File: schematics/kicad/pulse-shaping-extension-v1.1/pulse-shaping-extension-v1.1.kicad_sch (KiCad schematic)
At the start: 86 parts, among them J1 Conn_02x10_Odd_Even, J2 Conn_Coaxial, J3 Conn_Coaxial, J4 Conn_01x02_Pin, J5 Conn_01x02_Pin, J6 Conn_01x03_Pin, J7 Conn_Coaxial, U1 AD9102BCPZRL7, U2 ADM8829ARTZ-REEL7, U3 ADA4817-1ACP, U4 THS3091DDAR, X1 OB3225125MLDB6SI-00

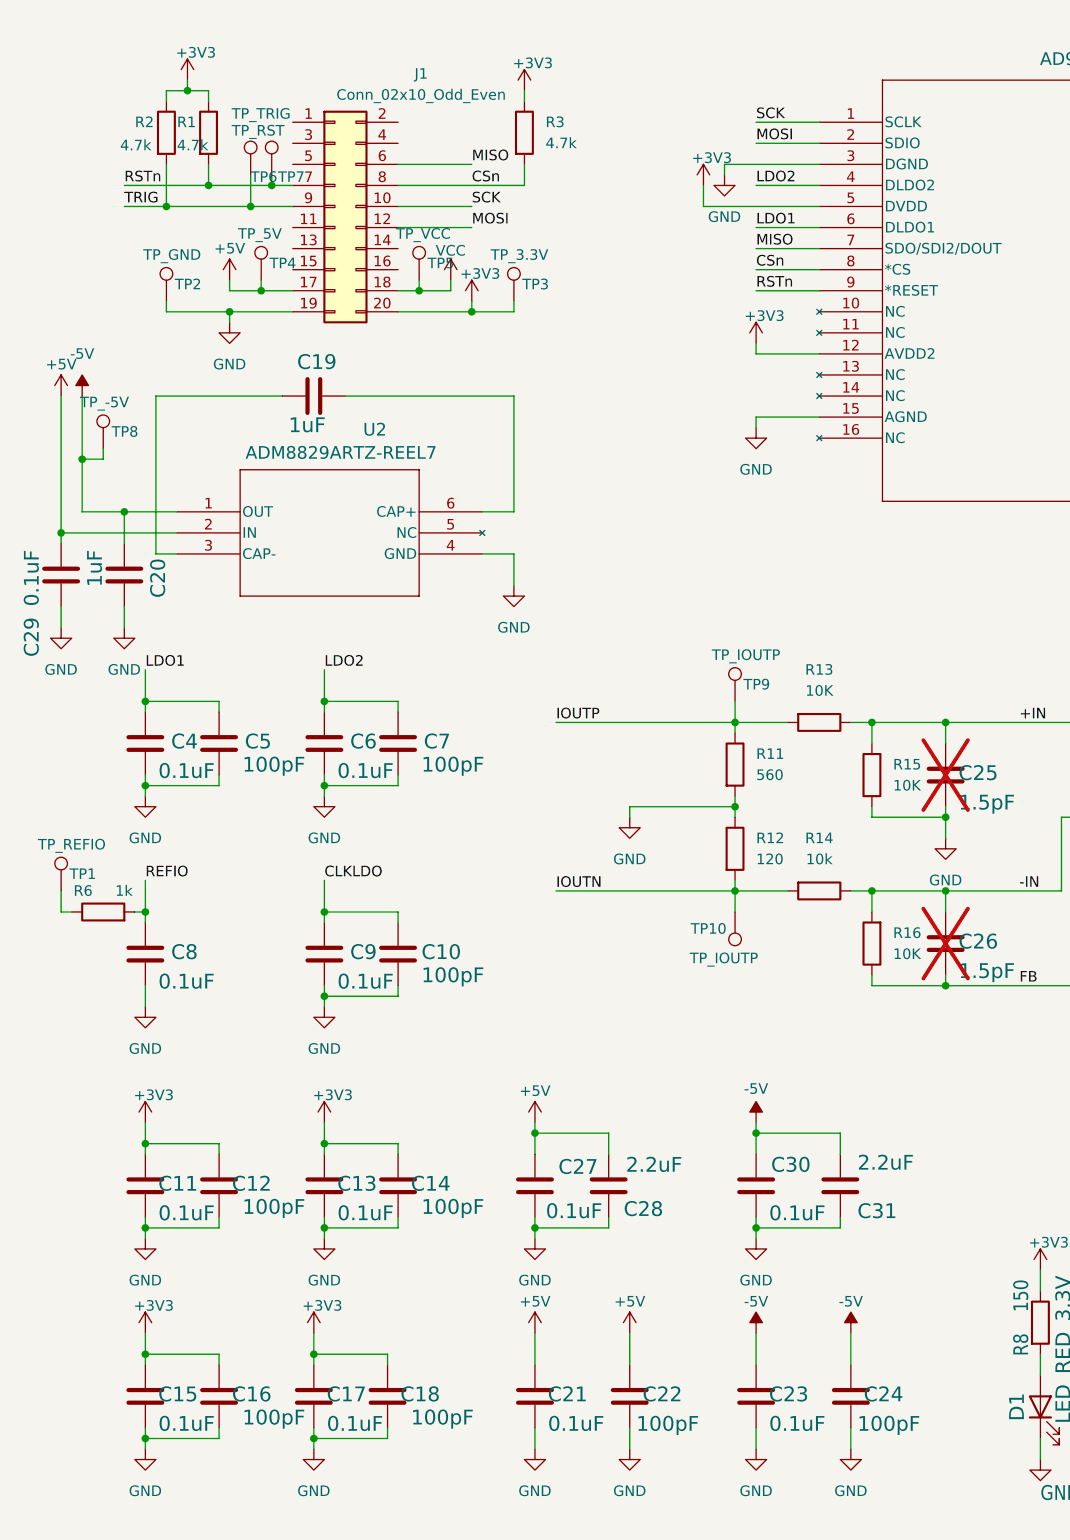
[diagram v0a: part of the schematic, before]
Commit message: Replaced dc-dc converter in pulse shaping expansion board.
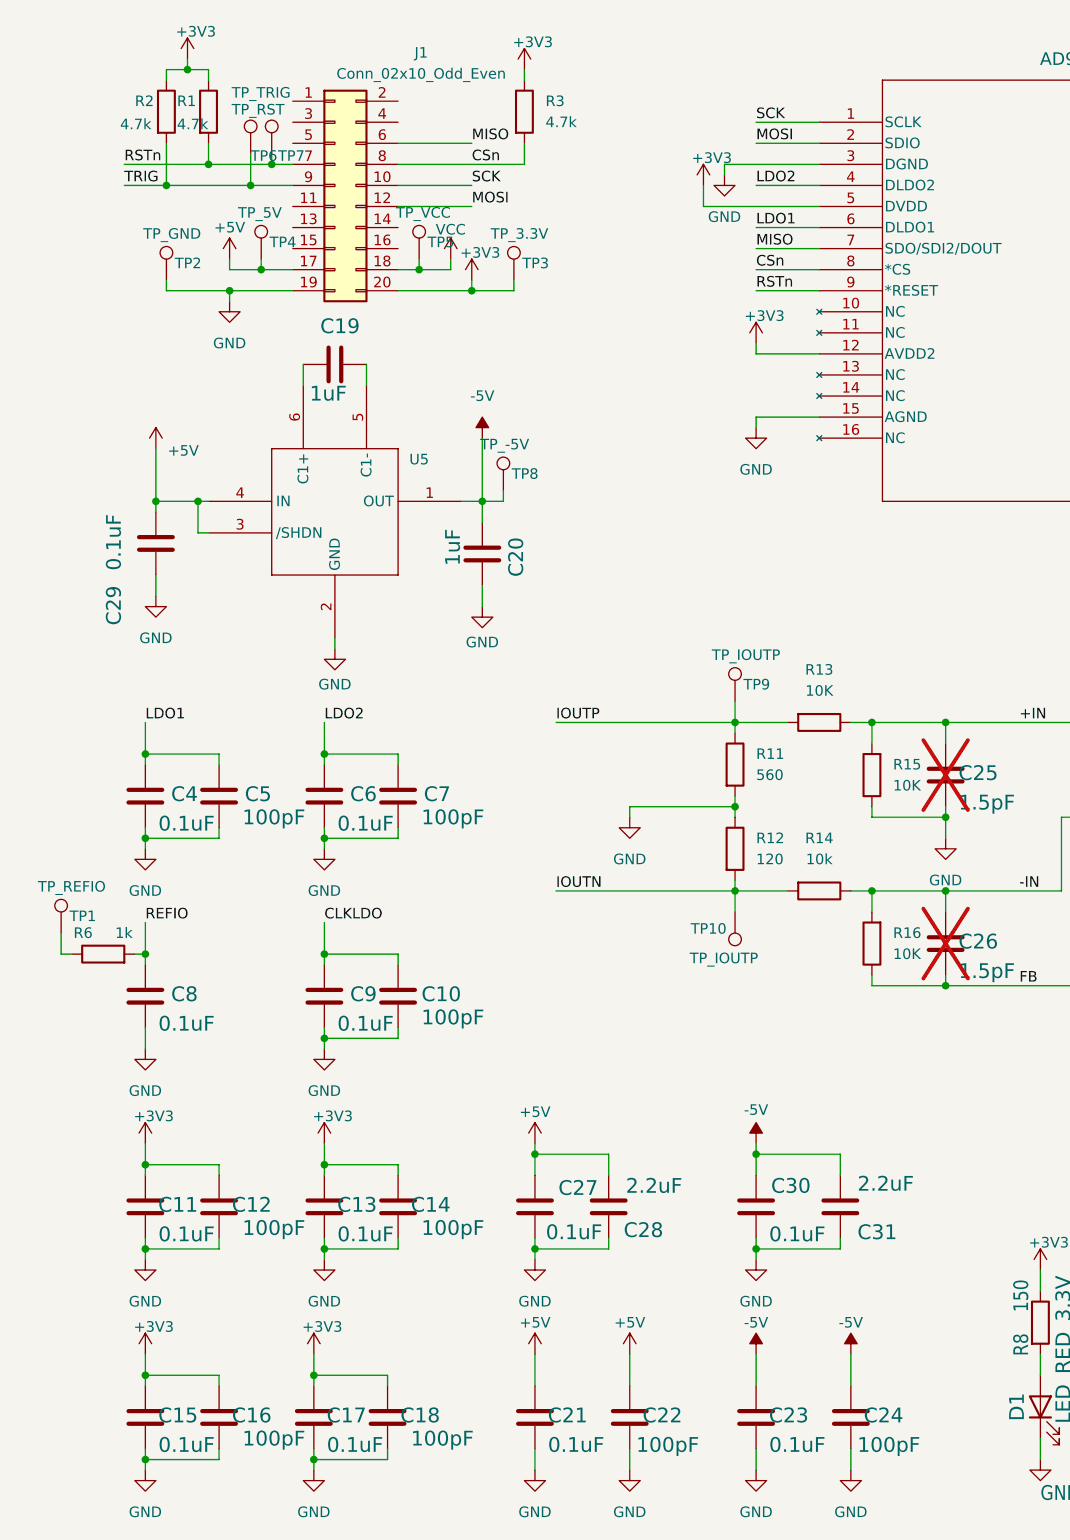
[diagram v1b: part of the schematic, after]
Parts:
- removed U2: ADM8829ARTZ-REEL7, RT_6_ADI, symbol adm8829:ADM8829ARTZ-REEL7
- added U5: ~, Package_TO_SOT_SMD:SOT-363_SC-70-6, symbol max1853ext:MAX1853EXT
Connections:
- net +5V: now also U5.3 (/SHDN), U5.4 (IN)
- net -5V: now also U5.1 (OUT)
- net GND: now also U5.2 (GND)
- net at C19.2: now also U5.6 (C1+)
- net at C19.1: now also U5.5 (C1-)
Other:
- moved on the sheet: C10, C11, C12, C13, C14, C15, C16, C17, C18, C19, C20, C21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
